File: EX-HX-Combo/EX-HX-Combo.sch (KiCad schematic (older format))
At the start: 45 parts, among them CN1 DB9 Male, J1 IDE_CONNECTOR, J200 Bus_Tandy_Plus_Through, J3 Bus_Tandy_Plus, SW1 SW_DIP_x10, U1 BIOS FLASH, U2 74HCT245, U3 1.8432 MHz, U4 DS1315, U5 AS6C4008-55PCN, U6 16550/16C550, U7 GD75232N, U8 GAL16V8, U9 GAL16V8, Y1 32.768 KHz

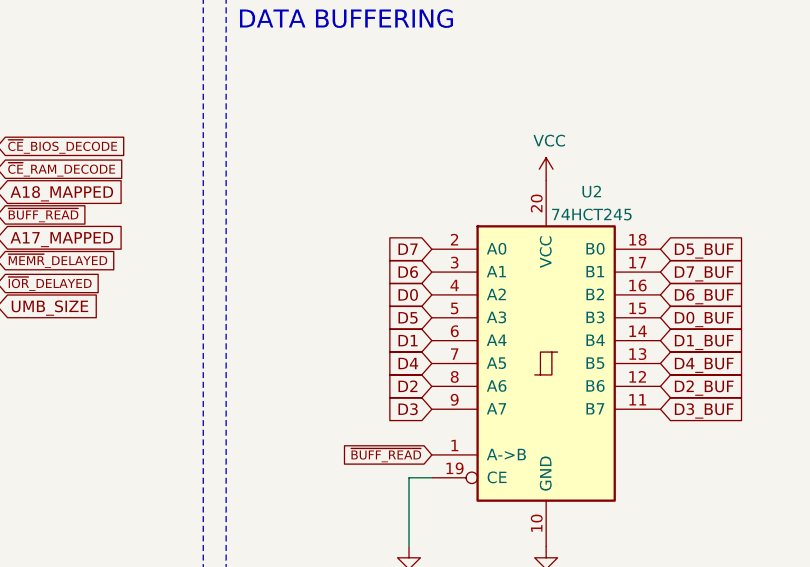
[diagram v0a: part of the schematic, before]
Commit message: EX-HX-Combo layout work.
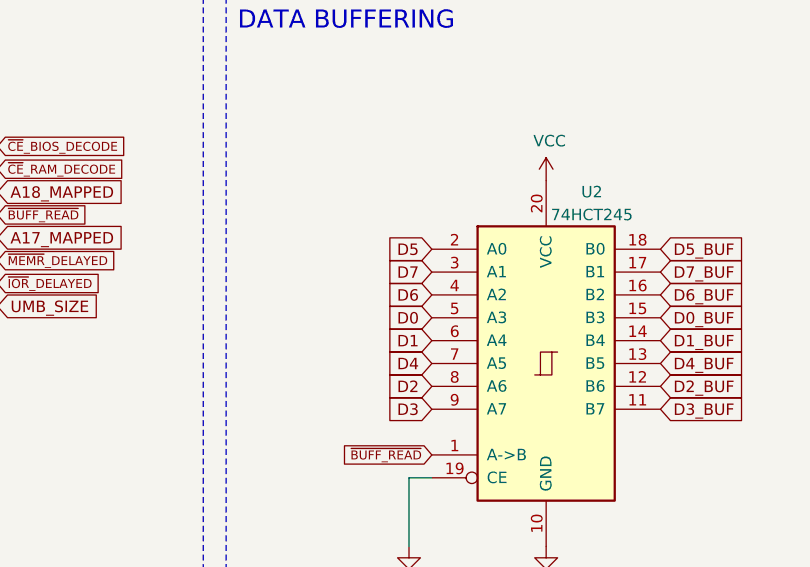
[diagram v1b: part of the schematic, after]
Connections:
- net D0: now also U2.5 (A3); no longer U2.4 (A2)
- net D5: now also U2.2 (A0); no longer U2.5 (A3)
- net D6: now also U2.4 (A2); no longer U2.3 (A1)
- net D7: now also U2.3 (A1); no longer U2.2 (A0)
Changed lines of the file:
@@
 Text GLabel 11100 2400 2    50   Input ~ 0
 D3_BUF
-Text GLabel 10100 1900 0    50   Input ~ 0
+Text GLabel 10100 2000 0    50   Input ~ 0
 D0
 Text GLabel 10100 2100 0    50   Input ~ 0
@@
 Text GLabel 10100 2200 0    50   Input ~ 0
 D4
-Text GLabel 10100 2000 0    50   Input ~ 0
+Text GLabel 10100 1700 0    50   Input ~ 0
 D5
+Text GLabel 10100 1900 0    50   Input ~ 0
+D6
 Text GLabel 10100 1800 0    50   Input ~ 0
-D6
-Text GLabel 10100 1700 0    50   Input ~ 0
 D7
 Text Notes 2350 11050 0    50   ~ 0
